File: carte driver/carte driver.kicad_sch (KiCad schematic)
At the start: 44 parts, among them J1 UART CP, J10 STEPPER 4, J11 STEPPER 3, J12 Conn_01x02, J3 UART BONUS, J4 Conn_01x02, J5 Conn_01x02, J6 STEPPER G, J7 STEPPER D, J8 STEPPER 1, J9 STEPPER 2, SW2 SW_DIP_x02, SW3 SW_DIP_x02, SW4 SW_DIP_x02, SW5 SW_DIP_x02, SW6 SW_DIP_x02, SW7 SW_DIP_x02, U1 TMC2209_SILENTSTEPSTICK, U10 XIAO-HALF-HOLE-23P, U2 TMC2209_SILENTSTEPSTICK, U3 TMC2209_SILENTSTEPSTICK, U4 TMC2209_SILENTSTEPSTICK, U5 TMC2209_SILENTSTEPSTICK, U6 TMC2209_SILENTSTEPSTICK

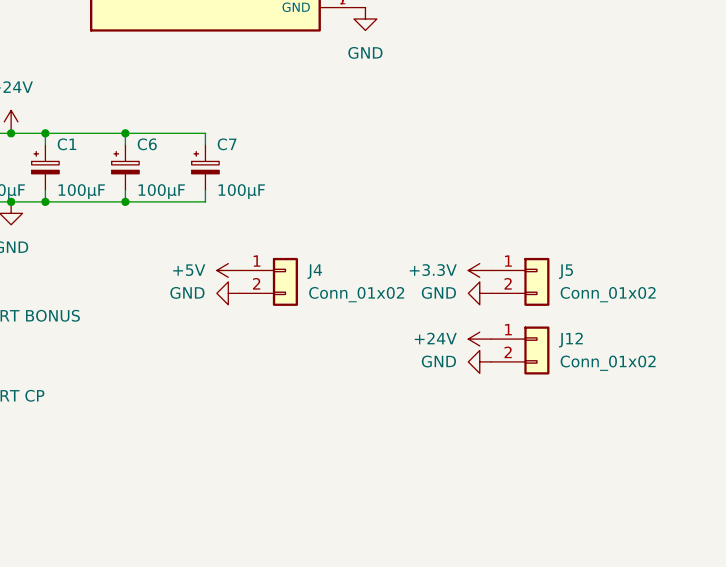
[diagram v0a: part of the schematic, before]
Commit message: boh il y a des trucs à changé ducoup
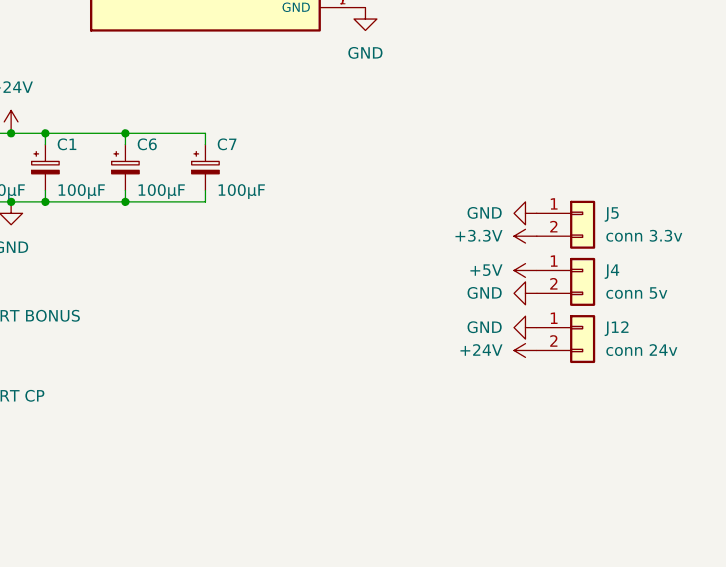
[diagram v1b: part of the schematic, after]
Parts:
- J12: value Conn_01x02 -> conn 24v
- J4: value Conn_01x02 -> conn 5v
- J5: value Conn_01x02 -> conn 3.3v
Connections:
- net +24V: now also J12.2 (Pin_2); no longer J12.1 (Pin_1)
- net +3.3V: now also J5.2 (Pin_2); no longer J5.1 (Pin_1)
- net GND: now also J12.1 (Pin_1), J5.1 (Pin_1); no longer J12.2 (Pin_2), J5.2 (Pin_2)
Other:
- moved on the sheet: J12, J4, J5
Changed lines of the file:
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@@
 	(symbol
 		(lib_id "power:+3.3V")
-		(at 240.03 142.24 90)
+		(at 245.11 138.43 90)
 		(unit 1)
 		(exclude_from_sim no)
@@
 		(fields_autoplaced yes)
 		(property "Reference" "#PWR015"
-			(at 243.84 142.24 0)
+			(at 248.92 138.43 0)
 			(effects
 				(font
@@
 		)
 		(property "Value" "+3.3V"
-			(at 236.22 142.2399 90)
+			(at 241.3 138.4299 90)
 			(effects
 				(font
@@
 		)
 		(property "Footprint" ""
-			(at 240.03 142.24 0)
+			(at 245.11 138.43 0)
 			(effects
 				(font
@@
 		)
 		(property "Datasheet" ""
-			(at 240.03 142.24 0)
+			(at 245.11 138.43 0)
 			(effects
 				(font
@@
 		)
 		(property "Description" "Power symbol creates a global label with name \"+3.3V\""
-			(at 240.03 142.24 0)
+			(at 245.11 138.43 0)
 			(effects
 				(font
@@
 		)
 		(instances
-			(project ""
+			(project "carte driver"
 				(path "/78588076-997a-4987-8ae5-538bbbdafc63"
 					(reference "#PWR015")
@@
 	(symbol
 		(lib_id "power:GND")
-		(at 240.03 144.78 270)
+		(at 245.11 135.89 270)
 		(unit 1)
 		(exclude_from_sim no)
@@
 		(fields_autoplaced yes)
 		(property "Reference" "#PWR04"
-			(at 233.68 144.78 0)
+			(at 238.76 135.89 0)
 			(effects
 				(font
@@
 		)
 		(property "Value" "GND"
-			(at 236.22 144.7799 90)
+			(at 241.3 135.8899 90)
 			(effects
 				(font
@@
 		)
 		(property "Footprint" ""
-			(at 240.03 144.78 0)
+			(at 245.11 135.89 0)
 			(effects
 				(font
@@
 		)
 		(property "Datasheet" ""
-			(at 240.03 144.78 0)
+			(at 245.11 135.89 0)
 			(effects
 				(font
@@
 		)
 		(property "Description" "Power symbol creates a global label with name \"GND\" , ground"
-			(at 240.03 144.78 0)
+			(at 245.11 135.89 0)
 			(effects
 				(font
@@
 		)
 		(instances
-			(project ""
+			(project "carte driver"
 				(path "/78588076-997a-4987-8ae5-538bbbdafc63"
 					(reference "#PWR04")
@@
 	(symbol
 		(lib_id "power:GND")
-		(at 212.09 144.78 270)
+		(at 245.11 144.78 270)
 		(unit 1)
 		(exclude_from_sim no)
@@
 		(fields_autoplaced yes)
 		(property "Reference" "#PWR016"
-			(at 205.74 144.78 0)
+			(at 238.76 144.78 0)
 			(effects
 				(font
@@
 		)
 		(property "Value" "GND"
-			(at 208.28 144.7799 90)
+			(at 241.3 144.7799 90)
 			(effects
 				(font
@@
 		)
 		(property "Footprint" ""
-			(at 212.09 144.78 0)
+			(at 245.11 144.78 0)
 			(effects
 				(font
@@
 		)
 		(property "Datasheet" ""
-			(at 212.09 144.78 0)
+			(at 245.11 144.78 0)
 			(effects
 				(font
@@
 		)
 		(property "Description" "Power symbol creates a global label with name \"GND\" , ground"
-			(at 212.09 144.78 0)
+			(at 245.11 144.78 0)
 			(effects
 				(font
@@
 	(symbol
 		(lib_id "power:GND")
-		(at 240.03 152.4 270)
+		(at 245.11 148.59 270)
 		(unit 1)
 		(exclude_from_sim no)
@@
 		(fields_autoplaced yes)
 		(property "Reference" "#PWR08"
-			(at 233.68 152.4 0)
+			(at 238.76 148.59 0)
 			(effects
 				(font
@@
 		)
 		(property "Value" "GND"
-			(at 236.22 152.3999 90)
+			(at 241.3 148.5899 90)
 			(effects
 				(font
@@
 		)
 		(property "Footprint" ""
-			(at 240.03 152.4 0)
+			(at 245.11 148.59 0)
 			(effects
 				(font
@@
 		)
 		(property "Datasheet" ""
-			(at 240.03 152.4 0)
+			(at 245.11 148.59 0)
 			(effects
 				(font
@@
 		)
 		(property "Description" "Power symbol creates a global label with name \"GND\" , ground"
-			(at 240.03 152.4 0)
+			(at 245.11 148.59 0)
 			(effects
 				(font
@@
 	(symbol
 		(lib_id "power:+24V")
-		(at 240.03 149.86 90)
+		(at 245.11 151.13 90)
 		(unit 1)
 		(exclude_from_sim no)
@@
 		(fields_autoplaced yes)
 		(property "Reference" "#PWR01"
-			(at 243.84 149.86 0)
+			(at 248.92 151.13 0)
 			(effects
 				(font
@@
 		)
 		(property "Value" "+24V"
-			(at 236.22 149.8599 90)
+			(at 241.3 151.1299 90)
 			(effects
 				(font
@@
 		)
 		(property "Footprint" ""
-			(at 240.03 149.86 0)
+			(at 245.11 151.13 0)
 			(effects
 				(font
@@
 		)
 		(property "Datasheet" ""
-			(at 240.03 149.86 0)
+			(at 245.11 151.13 0)
 			(effects
 				(font
@@
 		)
 		(property "Description" "Power symbol creates a global label with name \"+24V\""
-			(at 240.03 149.86 0)
+			(at 245.11 151.13 0)
 			(effects
 				(font
@@
 	(symbol
 		(lib_id "Connector_Generic:Conn_01x02")
-		(at 217.17 142.24 0)
+		(at 250.19 142.24 0)
 		(unit 1)
 		(exclude_from_sim no)
@@
 		(fields_autoplaced yes)
 		(property "Reference" "J4"
-			(at 219.71 142.2399 0)
+			(at 252.73 142.2399 0)
 			(effects
 				(font
@@
 			)
 		)
-		(property "Value" "Conn_01x02"
-			(at 219.71 144.7799 0)
+		(property "Value" "conn 5v"
+			(at 252.73 144.7799 0)
 			(effects
 				(font
@@
 		)
 		(property "Footprint" "Connector_Molex:Molex_KK-254_AE-6410-02A_1x02_P2.54mm_Vertical"
-			(at 217.17 142.24 0)
+			(at 250.19 142.24 0)
 			(effects
 				(font
@@
 		)
 		(property "Datasheet" "~"
-			(at 217.17 142.24 0)
+			(at 250.19 142.24 0)
 			(effects
 				(font
@@
 		)
 		(property "Description" "Generic connector, single row, 01x02, script generated (kicad-library-utils/schlib/autogen/connector/)"
-			(at 217.17 142.24 0)
+			(at 250.19 142.24 0)
 			(effects
 				(font
@@
 	(symbol
 		(lib_id "Connector_Generic:Conn_01x02")
-		(at 245.11 149.86 0)
+		(at 250.19 148.59 0)
 		(unit 1)
 		(exclude_from_sim no)
@@
 		(fields_autoplaced yes)
 		(property "Reference" "J12"
-			(at 247.65 149.8599 0)
+			(at 252.73 148.5899 0)
 			(effects
 				(font
@@
 			)
 		)
-		(property "Value" "Conn_01x02"
-			(at 247.65 152.3999 0)
+		(property "Value" "conn 24v"
+			(at 252.73 151.1299 0)
 			(effects
 				(font
@@
 		)
 		(property "Footprint" "Connector_AMASS:AMASS_XT60-F_1x02_P7.20mm_Vertical"
-			(at 245.11 149.86 0)
+			(at 250.19 148.59 0)
 			(effects
 				(font
@@
 		)
 		(property "Datasheet" "~"
-			(at 245.11 149.86 0)
+			(at 250.19 148.59 0)
 			(effects
 				(font
@@
 		)
 		(property "Description" "Generic connector, single row, 01x02, script generated (kicad-library-utils/schlib/autogen/connector/)"
-			(at 245.11 149.86 0)
+			(at 250.19 148.59 0)
 			(effects
 				(font
@@
 	(symbol
 		(lib_id "power:+5V")
-		(at 212.09 142.24 90)
+		(at 245.11 142.24 90)
 		(unit 1)
 		(exclude_from_sim no)
@@
 		(fields_autoplaced yes)
 		(property "Reference" "#PWR02"
-			(at 215.9 142.24 0)
+			(at 248.92 142.24 0)
 			(effects
 				(font
@@
 		)
 		(property "Value" "+5V"
-			(at 208.28 142.2399 90)
+			(at 241.3 142.2399 90)
 			(effects
 				(font
@@
 		)
 		(property "Footprint" ""
-			(at 212.09 142.24 0)
+			(at 245.11 142.24 0)
 			(effects
 				(font
@@
 		)
 		(property "Datasheet" ""
-			(at 212.09 142.24 0)
+			(at 245.11 142.24 0)
 			(effects
 				(font
@@
 		)
 		(property "Description" "Power symbol creates a global label with name \"+5V\""
-			(at 212.09 142.24 0)
+			(at 245.11 142.24 0)
 			(effects
 				(font
@@
 	(symbol
 		(lib_id "Connector_Generic:Conn_01x02")
-		(at 245.11 142.24 0)
+		(at 250.19 135.89 0)
 		(unit 1)
 		(exclude_from_sim no)
@@
 		(fields_autoplaced yes)
 		(property "Reference" "J5"
-			(at 247.65 142.2399 0)
+			(at 252.73 135.8899 0)
 			(effects
 				(font
@@
 			)
 		)
-		(property "Value" "Conn_01x02"
-			(at 247.65 144.7799 0)
+		(property "Value" "conn 3.3v"
+			(at 252.73 138.4299 0)
 			(effects
 				(font
@@
 		)
 		(property "Footprint" "Connector_AMASS:AMASS_XT30U-F_1x02_P5.0mm_Vertical"
-			(at 245.11 142.24 0)
+			(at 250.19 135.89 0)
 			(effects
 				(font
@@
 		)
 		(property "Datasheet" "~"
-			(at 245.11 142.24 0)
+			(at 250.19 135.89 0)
 			(effects
 				(font
@@
 		)
 		(property "Description" "Generic connector, single row, 01x02, script generated (kicad-library-utils/schlib/autogen/connector/)"
-			(at 245.11 142.24 0)
+			(at 250.19 135.89 0)
 			(effects
 				(font
